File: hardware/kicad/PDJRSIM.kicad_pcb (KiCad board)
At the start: 2 copper layers, 100 x 85 mm, 110 parts, among them J1 Screw_Terminal_01x09, J101 CAN, J2 Screw_Terminal_01x09, Q101 BSS138, Q102 BSS138, SW101 BUS, SW102 ADDR/VALUE, SW103 PRG, U1 BCR401, U10 BCR401 (16x), U101 TMR-2-2411, U102 MCP2551-I-P, U103 Teensy_4.0, U104 74HC165, U105 74HCT595, U11 BCR401 (16x), U12 BCR401 (16x), U13 BCR401 (16x), U14 ASCL-6400, U15 BCR401 (16x), U16 BCR401 (16x), U17 74LS165, U18 BCR401 (16x), U19 BCR401 (16x), U2 BCR401, U20 ASCL-6400, U21 BCR401 (16x), U22 BCR401 (16x), U3 ASCL-6400, U4 BCR401, U5 BCR401 (16x), U6 74LS165, U7 BCR401 (16x), U8 BCR401 (16x), U9 ASCL-6400

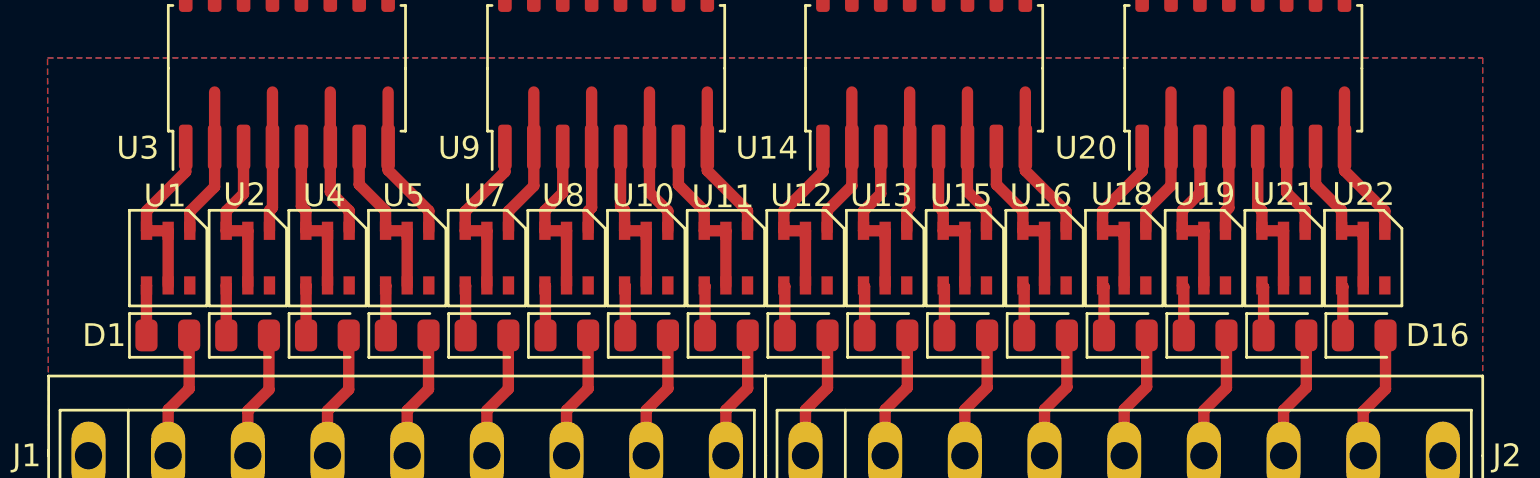
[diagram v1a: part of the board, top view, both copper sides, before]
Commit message: Fix a break
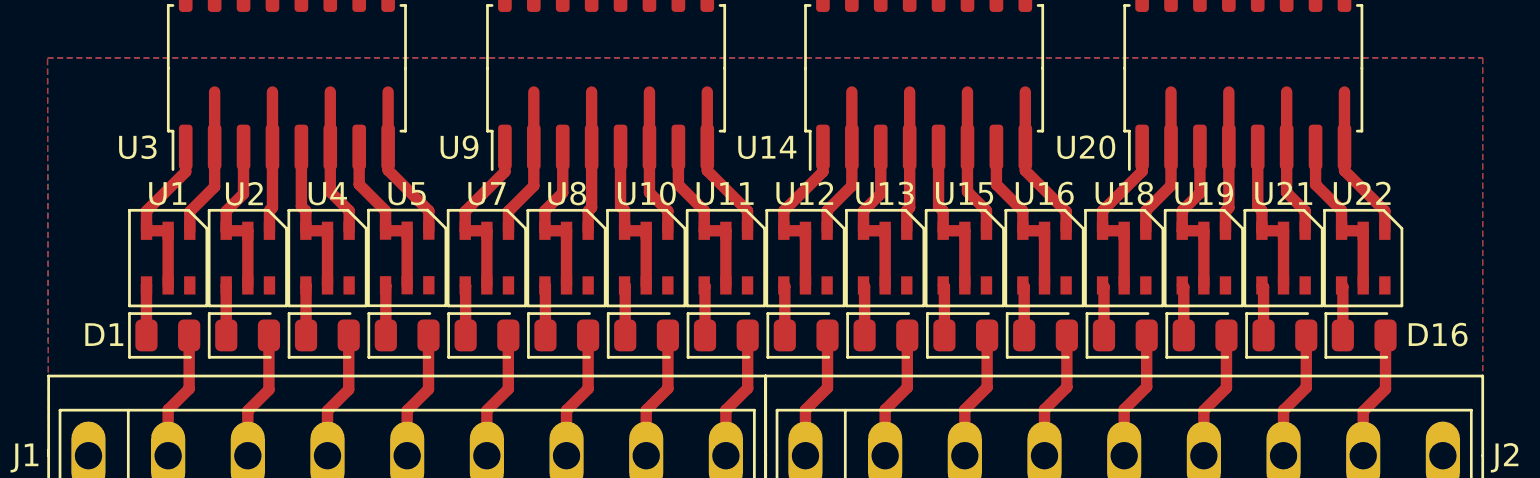
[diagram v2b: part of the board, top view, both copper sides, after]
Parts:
- U10, U11, U12, U13, U15, U16, U18, U19, U21, U22, U5, U7, U8: value BCR401 (16x) -> BCR401
